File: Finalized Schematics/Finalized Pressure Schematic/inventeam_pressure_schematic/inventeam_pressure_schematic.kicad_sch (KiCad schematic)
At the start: 5 parts, among them J1 Conn_02x20_Top_Bottom

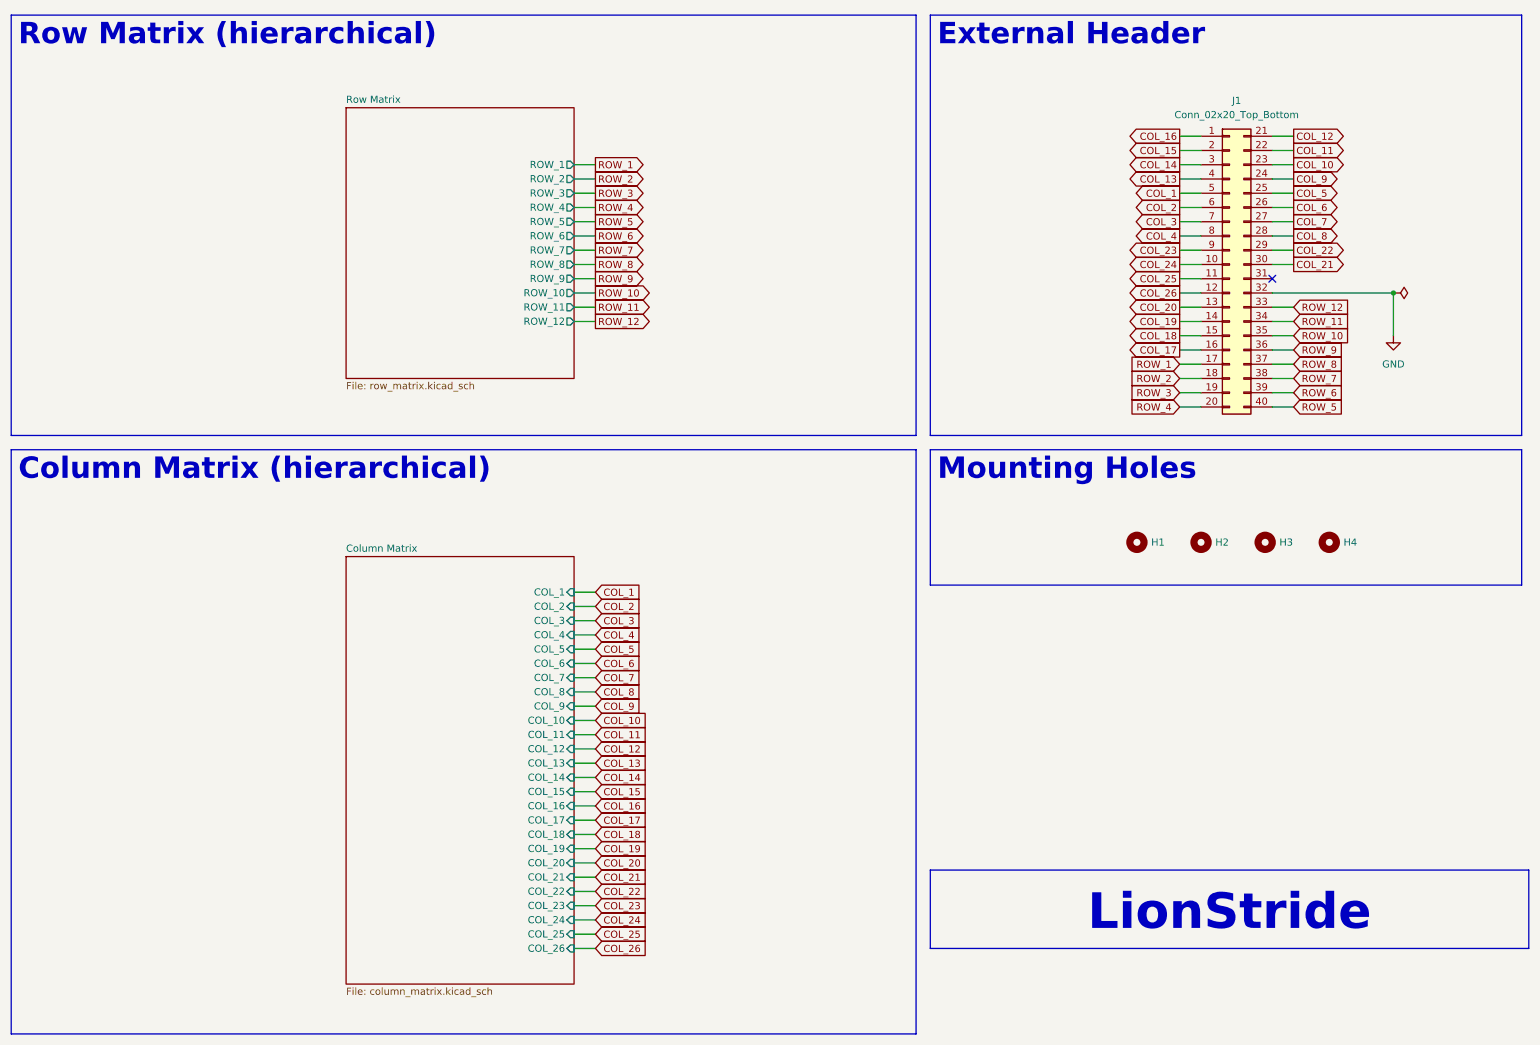
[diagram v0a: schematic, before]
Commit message: Pressure V2.1
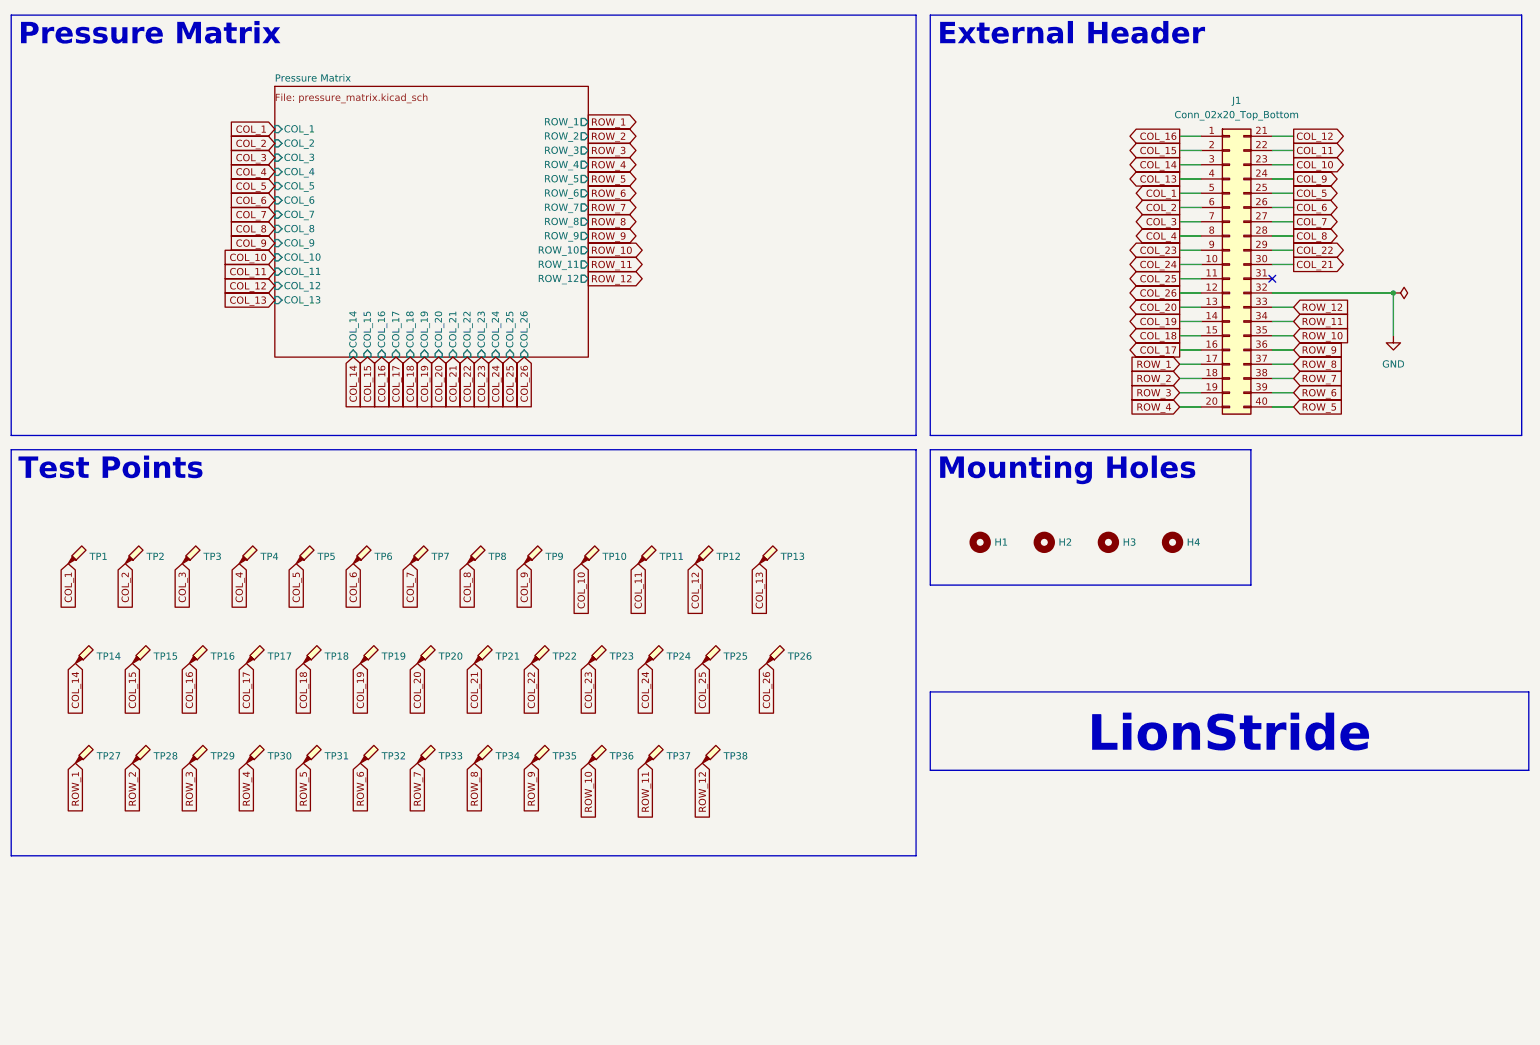
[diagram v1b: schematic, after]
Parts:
- added TP1, TP10, TP11, TP12, TP13, TP14, TP15, TP16, TP17, TP18, TP19, TP2, TP20, TP21, TP22, TP23, TP24, TP25, TP26, TP27, TP28, TP29, TP3, TP30, TP31, TP32, TP33, TP34, TP35, TP36, TP37, TP38, TP4, TP5, TP6, TP7, TP8, TP9: TestPoint_Probe, TestPoint:TestPoint_Pad_D2.5mm, symbol Connector:TestPoint_Probe
- H1, H2, H3, H4: footprint (none) -> MountingHole:MountingHole_2.7mm_M2.5
- J1: footprint (none) -> Connector_PinHeader_2.54mm:PinHeader_2x20_P2.54mm_Vertical
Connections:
- net COL_1: now also TP1.1
- net COL_10: now also TP10.1
- net COL_11: now also TP11.1
- net COL_12: now also TP12.1
- net COL_13: now also TP13.1
- net COL_14: now also TP14.1
- net COL_15: now also TP15.1
- net COL_16: now also TP16.1
- net COL_17: now also TP17.1
- net COL_18: now also TP18.1
- net COL_19: now also TP19.1
- net COL_2: now also TP2.1
- net COL_20: now also TP20.1
- net COL_21: now also TP21.1
- net COL_22: now also TP22.1
- net COL_23: now also TP23.1
- net COL_24: now also TP24.1
- net COL_25: now also TP25.1
- net COL_26: now also TP26.1
- net COL_3: now also TP3.1
- net COL_4: now also TP4.1
- net COL_5: now also TP5.1
- net COL_6: now also TP6.1
- net COL_7: now also TP7.1
- net COL_8: now also TP8.1
- net COL_9: now also TP9.1
- net ROW_1: now also TP27.1
- net ROW_10: now also TP36.1
- net ROW_11: now also TP37.1
- net ROW_12: now also TP38.1
- net ROW_2: now also TP28.1
- net ROW_3: now also TP29.1
- net ROW_4: now also TP30.1
- net ROW_5: now also TP31.1
- net ROW_6: now also TP32.1
- net ROW_7: now also TP33.1
- net ROW_8: now also TP34.1
- net ROW_9: now also TP35.1
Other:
- sheet Row Matrix renamed Pressure Matrix
- removed sheet Column Matrix
- sheet Pressure Matrix: file row_matrix.kicad_sch -> pressure_matrix.kicad_sch
- sheet Pressure Matrix ports: added COL_1, COL_10, COL_11, COL_12, COL_13, COL_14, COL_15, COL_16, COL_17, COL_18, COL_19, COL_2, COL_20, COL_21, COL_22, COL_23, COL_24, COL_25, COL_26, COL_3, COL_4, COL_5, COL_6, COL_7, COL_8, COL_9; removed none
- note added: "Pressure Matrix"
- note added: "Test Points"
- note removed: "Column Matrix (hierarchical)"
- note removed: "Row Matrix (hierarchical)"
- moved on the sheet: H1, H2, H3, H4
